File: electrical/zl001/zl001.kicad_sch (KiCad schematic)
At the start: 1 part

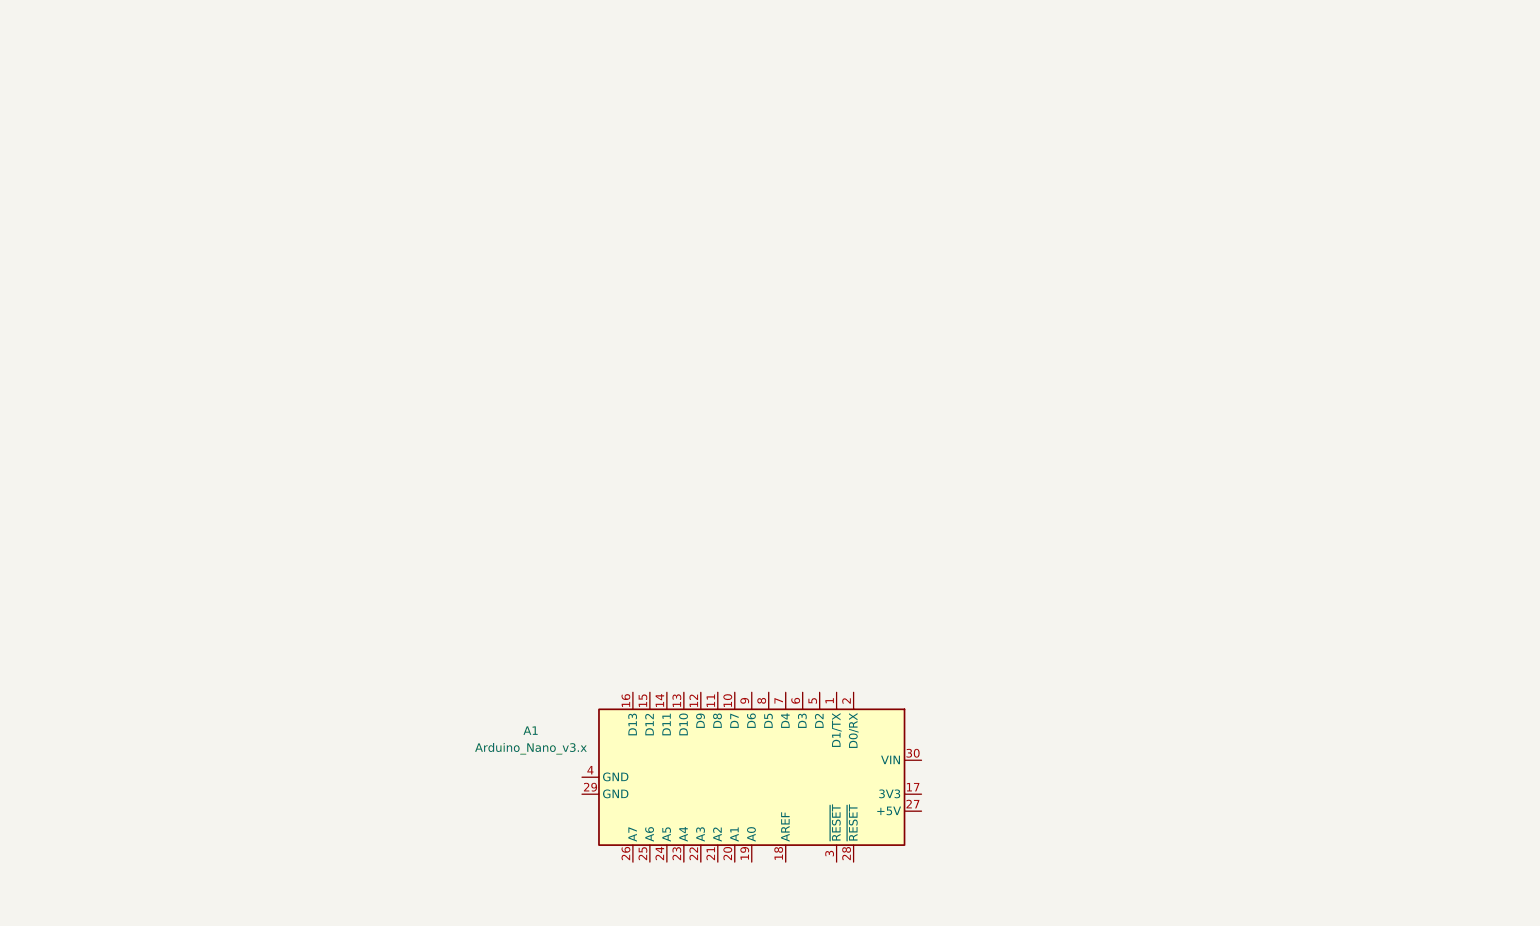
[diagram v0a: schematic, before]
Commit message: v0.01
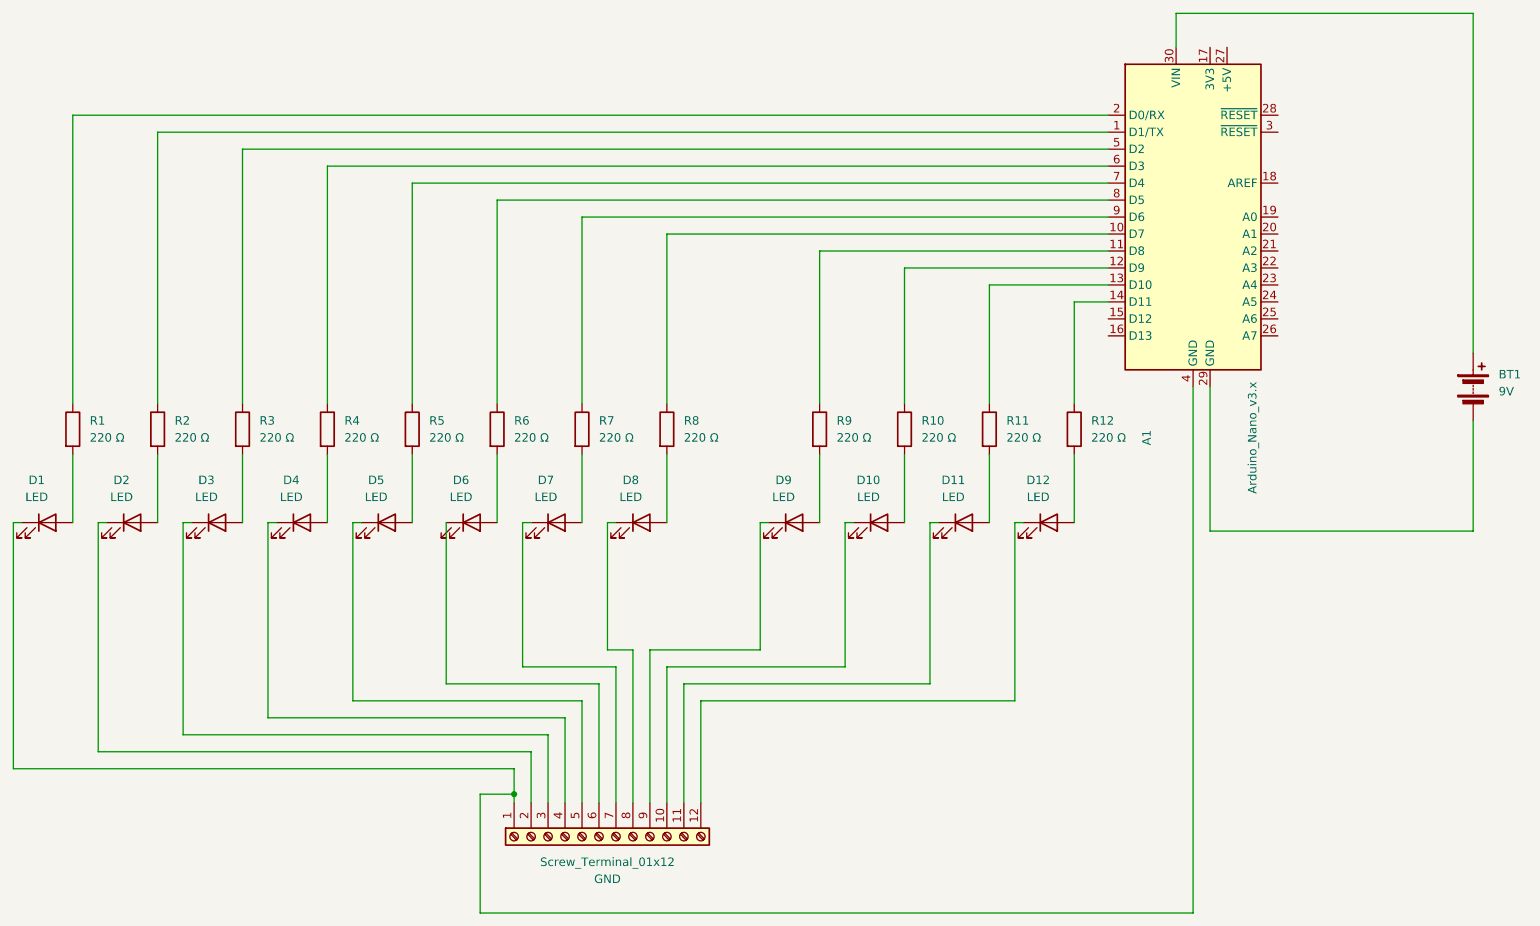
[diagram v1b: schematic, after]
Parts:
- added BT1: 9V, symbol Device:Battery
- added D1, D10, D11, D12, D2, D3, D4, D5, D6, D7, D8, D9: LED, symbol Device:LED
- added GND: Screw_Terminal_01x12, symbol Connector:Screw_Terminal_01x12
- added R1, R10, R11, R12, R2, R3, R4, R5, R6, R7, R8, R9: 220 Ω, symbol Device:R
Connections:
- net at A1.1 (D1/TX): now also R2.1
- net at A1.10 (D7): now also R8.1
- net at A1.11 (D8): now also R9.1
- net at A1.12 (D9): now also R10.1
- net at A1.13 (D10): now also R11.1
- net at A1.14 (D11): now also R12.1
- net at A1.2 (D0/RX): now also R1.1
- net at A1.29 (GND): now also BT1.2 (-)
- net at A1.30 (VIN): now also BT1.1 (+)
- net at A1.4 (GND): now also D1.1 (K), GND.1 (Pin_1)
- net at A1.5 (D2): now also R3.1
- net at A1.6 (D3): now also R4.1
- net at A1.7 (D4): now also R5.1
- net at A1.8 (D5): now also R6.1
- net at A1.9 (D6): now also R7.1
- new net: D10.1 (K), GND.10 (Pin_10)
- new net: D10.2 (A), R10.2
- new net: D7.1 (K), GND.7 (Pin_7)
- new net: D7.2 (A), R7.2
- new net: D4.1 (K), GND.4 (Pin_4)
- new net: D4.2 (A), R4.2
- new net: D3.1 (K), GND.3 (Pin_3)
- new net: D3.2 (A), R3.2
- new net: D11.1 (K), GND.11 (Pin_11)
- new net: D11.2 (A), R11.2
- new net: D2.1 (K), GND.2 (Pin_2)
- new net: D2.2 (A), R2.2
- new net: D5.1 (K), GND.5 (Pin_5)
- new net: D5.2 (A), R5.2
- new net: D12.1 (K), GND.12 (Pin_12)
- new net: D6.1 (K), GND.6 (Pin_6)
- new net: D8.1 (K), GND.8 (Pin_8)
- new net: D9.1 (K), GND.9 (Pin_9)
- new net: D12.2 (A), R12.2
- new net: D1.2 (A), R1.2
- new net: D8.2 (A), R8.2
- new net: D9.2 (A), R9.2
- new net: D6.2 (A), R6.2
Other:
- moved on the sheet: A1
